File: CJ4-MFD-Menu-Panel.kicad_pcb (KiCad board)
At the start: 2 copper layers, 122.4 x 62.5 mm, 77 parts, among them J1 USB_B_Mini, J2 AVR-ISP-6, SW1 SW_Push_LED, SW10 5_Way_Switch, SW11 SW_Push_LED, SW12 SW_Push_LED, SW13 SW_Push_LED, SW14 SW_Push_LED, SW15 SW_Push_LED, SW16 SW_Push_LED, SW17 SW_Push_LED, SW18 SW_Push_LED, SW19 SW_Push_LED, SW2 SW_Push_LED, SW20 SW_Push_LED, SW21 SW_Push_LED, SW3 SW_Push_LED, SW4 SW_Push_LED, SW5 SW_Push_LED, SW6 SW_Push_LED, SW7 SW_Push_LED, SW8 SW_Push_LED, SW9 SW_Push_LED, U1 MCP23017_SO, U2 MCP23017_SO, U3 IS31FL3733B, U4 ATmega32U4RC-MU, Y1 16MHz

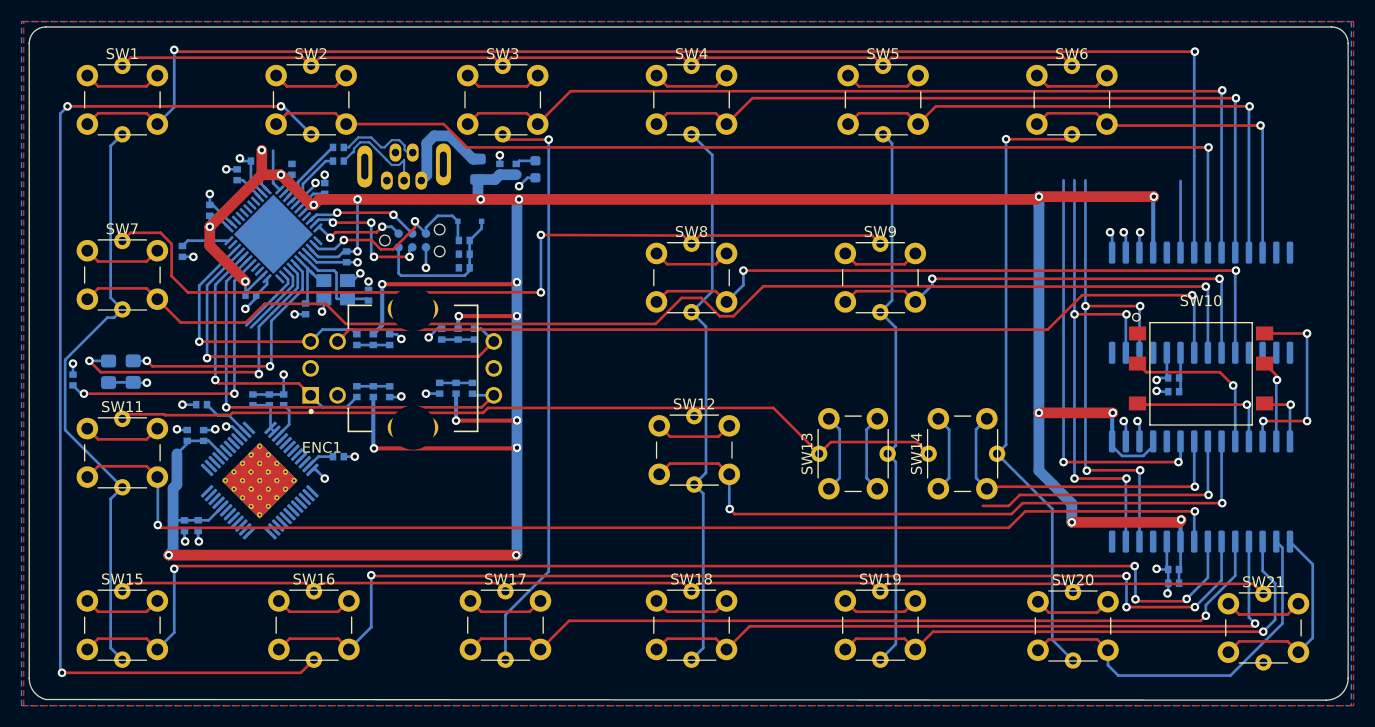
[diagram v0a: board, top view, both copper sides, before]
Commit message: Fully routed and ready to go
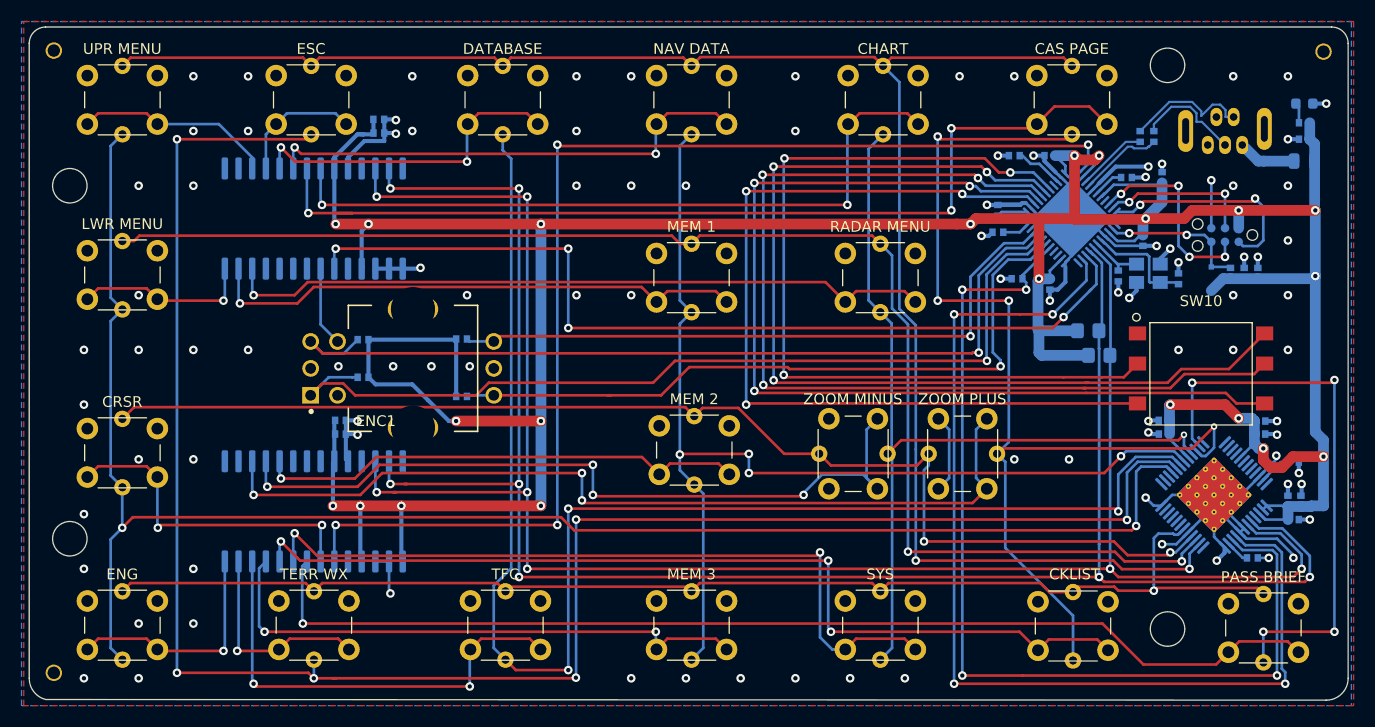
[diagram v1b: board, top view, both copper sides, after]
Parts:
- removed C1, C2, C3, C4: 0.01uf, CJ4-MFD-Menu-Panel:Perfect_0402
- removed R5, R6, R7, R8: 10k, CJ4-MFD-Menu-Panel:Perfect_0402
- added H1: MountingHole, MountingHole:MountingHole_3.2mm_M3, F.Cu at (34.2, 35.6)
- added H2: MountingHole, MountingHole:MountingHole_3.2mm_M3, F.Cu at (34.2, 68.3)
- added H3: MountingHole, MountingHole:MountingHole_3.2mm_M3, F.Cu at (136.1, 24.4)
- added H4: MountingHole, MountingHole:MountingHole_3.2mm_M3, F.Cu at (136.1, 76.7)
- added H5: JLCPCB, CJ4-MFD-Menu-Panel:JLCPCB_Tooling_Hole, F.Cu at (32.8, 23.1)
- added H6: JLCPCB, CJ4-MFD-Menu-Panel:JLCPCB_Tooling_Hole, F.Cu at (150.6, 23.2)
- added H7: JLCPCB, CJ4-MFD-Menu-Panel:JLCPCB_Tooling_Hole, F.Cu at (32.8, 80.9)
- moved R10 101.5 mm to (147.8, 61.2), turned to 0 degrees
- moved C12 99.6 mm to (144.7, 57.4), turned to 0 degrees
- moved C11 98.0 mm to (144.7, 58.6), turned to 0 degrees
- moved C14 96.5 mm to (147.3, 64.8)
- moved C13 96.2 mm to (148.5, 64.8)
- moved C15 94.4 mm to (147.8, 66.5), turned to 0 degrees
- moved C9 91.5 mm to (135.8, 57.3), turned to 180 degrees
- moved R17 91.0 mm to (128.8, 49.0), turned to 180 degrees
- moved C10 90.1 mm to (135.8, 58.6), turned to 180 degrees
- moved R16 89.7 mm to (129.8, 51.3), turned to 0 degrees
- moved U3 88.6 mm to (140.5, 64.3), turned to 45 degrees
- moved R19 88.1 mm to (122.2, 44.2), turned to 180 degrees
- moved C7 85.4 mm to (62.9, 29.4), turned to 0 degrees
- moved R9 85.4 mm to (144.0, 70.1)
- moved C8 84.2 mm to (62.9, 30.7), turned to 0 degrees
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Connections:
- U1 pad 21: UPR_MENU -> E_BTN
- U1 pad 22: ESC -> Net-(U1-Pad22)
- U1 pad 23: DATABASE -> Net-(U1-Pad23)
- U1 pad 24: NAV_DATA -> Net-(U1-Pad24)
- U1 pad 25: CHART -> Net-(U1-Pad25)
- U1 pad 26: CAS_PAGE -> RADAR_MENU
- U1 pad 27: Net-(U1-Pad27) -> MEM_1
- U1 pad 28: Net-(U1-Pad28) -> LWR_MENU
- U1 pad 3: Net-(U1-Pad3) -> UPR_MENU
- U1 pad 4: Net-(U1-Pad4) -> ESC
- U1 pad 5: MEM_1 -> DATABASE
- U1 pad 6: RADAR_MENU -> NAV_DATA
- U1 pad 7: LWR_MENU -> CAS_PAGE
- U1 pad 8: E_BTN -> CHART
- U2 pad 1: PASS_BRIEF -> Net-(U2-Pad1)
- U2 pad 2: CKLIST -> Net-(U2-Pad2)
- U2 pad 21: ZOOM_PLUS -> CRSR
- U2 pad 22: ZOOM_MINUS -> PASS_BRIEF
- U2 pad 23: MEM_2 -> SYS
- U2 pad 24: LEFT -> CKLIST
- U2 pad 25: CTR -> MEM_3
- U2 pad 26: DOWN -> TFC
- U2 pad 27: RIGHT -> TERR_WX
- U2 pad 28: UP -> ENG
- U2 pad 3: SYS -> ZOOM_PLUS
- U2 pad 4: MEM_3 -> ZOOM_MINUS
- U2 pad 5: TFC -> MEM_2
- U2 pad 6: TERR_WX -> Net-(U2-Pad6)
- U2 pad 7: ENG -> Net-(U2-Pad7)
- U2 pad 8: CRSR -> Net-(U2-Pad8)
- U4 pad 30: B -> B'
- U4 pad 31: B' -> B
- U4 pad 36: Net-(U4-Pad36) -> CTR
- U4 pad 37: Net-(U4-Pad37) -> UP
- U4 pad 38: Net-(U4-Pad38) -> RIGHT
- U4 pad 39: Net-(U4-Pad39) -> DOWN
- U4 pad 40: Net-(U4-Pad40) -> LEFT
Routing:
- net UPR_MENU: track 128.4 -> 18.6 mm, vias 2 -> 0
- net SCL: track 72.1 -> 178.8 mm, vias 6 -> 7
- net SDA: track 76.5 -> 178.4 mm, vias 6 -> 7
- net CS1: track 55.3 -> 155.5 mm, vias 0 -> 2
- net LWR_MENU: track 116.1 -> 16.5 mm
- net ENG: track 118.9 -> 21.9 mm, vias 4 -> 1
- net LED_INTB: track 6.47 -> 97.9 mm, vias 0 -> 4
- net UP: track 5.91 -> 94.2 mm, vias 1 -> 3
- net RIGHT: track 7.73 -> 94.2 mm, vias 1 -> 3
- net ESC: track 98.1 -> 11.8 mm, vias 1 -> 0
- net PASS_BRIEF: track 19.0 -> 101.3 mm, vias 0 -> 1
- net TERR_WX: track 101.6 -> 19.6 mm, vias 4 -> 1
- net CRSR: track 111.6 -> 30.8 mm
- net E_BTN: track 86.5 -> 7.41 mm, vias 1 -> 0
- net CS3: track 54.4 -> 132.9 mm, vias 1 -> 3
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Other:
- board text added: "%%version%% %%date%%"
- board text added: "CAS PAGE"
- board text added: "CHART"
- board text added: "CJ4 MFD panel Neil Enns neile@live.com"
- board text added: "CKLIST"
- board text added: "CRSR"
- board text added: "DATABASE"
- board text added: "ENG"
- board text added: "ESC"
- board text added: "JLCJLCJLCJLC"
- board text added: "LWR MENU"
- board text added: "MEM 1"
- board text added: "MEM 2"
- board text added: "MEM 3"
- board text added: "NAV DATA"
- board text added: "PASS BRIEF"
- board text added: "RADAR MENU"
- board text added: "SYS"
- board text added: "TERR WX"
- board text added: "TFC"
- board text added: "UPR MENU"
- board text added: "ZOOM MINUS"
- board text added: "ZOOM PLUS"
